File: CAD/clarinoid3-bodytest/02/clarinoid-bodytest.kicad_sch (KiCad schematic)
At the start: 10 parts, among them J13 clarinoid3 main usb interconn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, J17 clarinoid3 main usb interconn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, SW1 sw_batteryindicator, SW6 sw_program, U17 OLED graphic

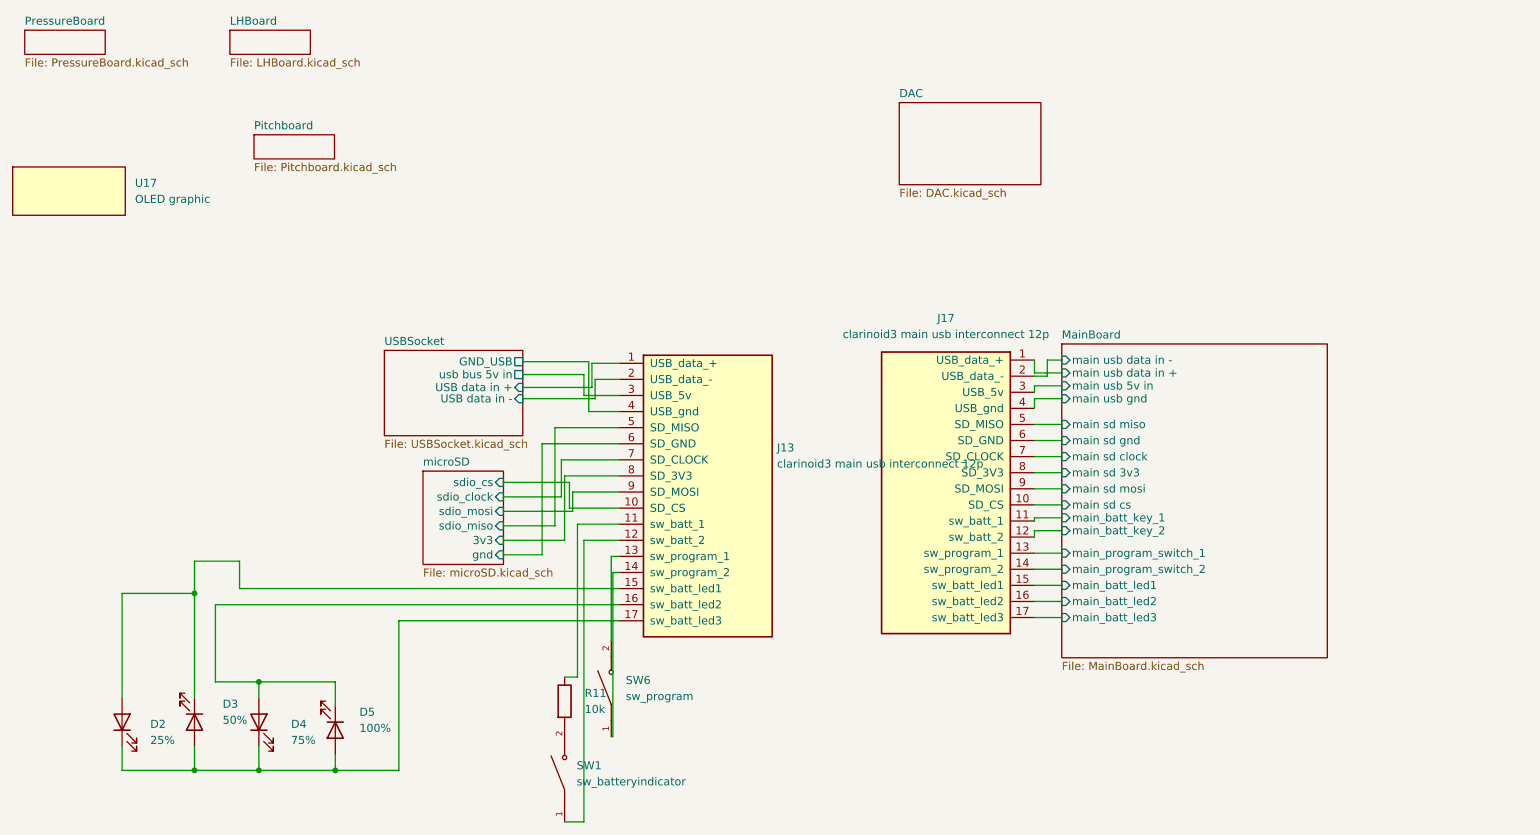
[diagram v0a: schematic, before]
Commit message: created clarinoid presets for Cave Bouncer more clarinoid3 pcb WIP midi performer application WIP; transitioning to Teensy4
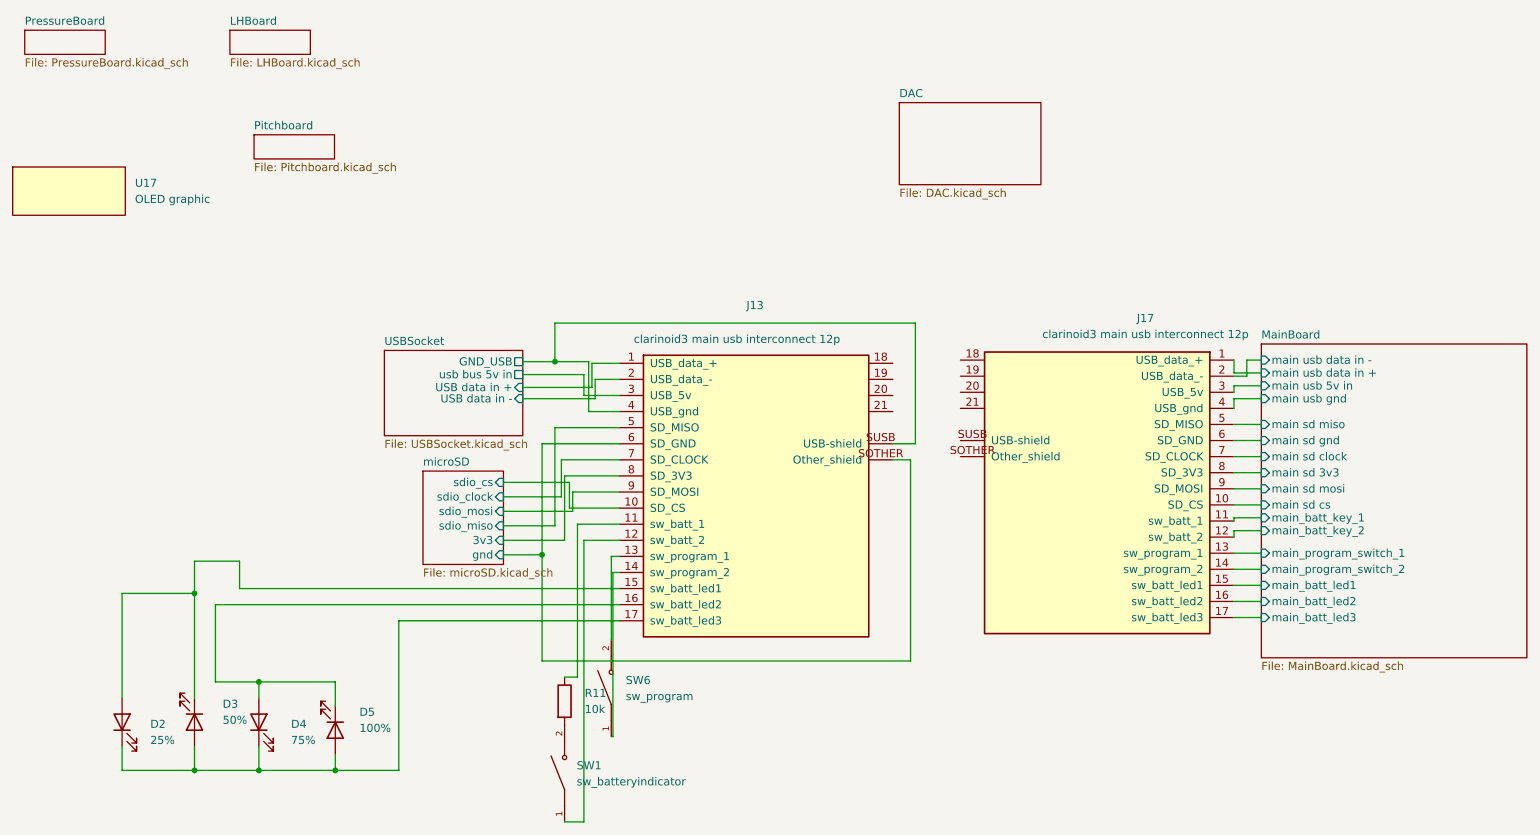
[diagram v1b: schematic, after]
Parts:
- J13: footprint clarinoid2:clarinoid 3 main sd interconnect castellated interconnect 17p -> clarinoid2:clarinoid3-sd subboard castellated
- J17: footprint clarinoid2:clarinoid 3 main sd interconnect SM interconnect 17p -> clarinoid2:clarinoid3-sd subboard smd
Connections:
- net USBSocket/GND_USB: now also J13.SUSB (USB-shield)
- net microSD/gnd: now also J13.SOTHER (Other_shield)
